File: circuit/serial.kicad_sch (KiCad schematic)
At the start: 21 parts, among them J1 Port B, J2 Port C, J4 Port A, J4 Port G, Q1 2N3904, Q2 2N3906, Q3 2N3906

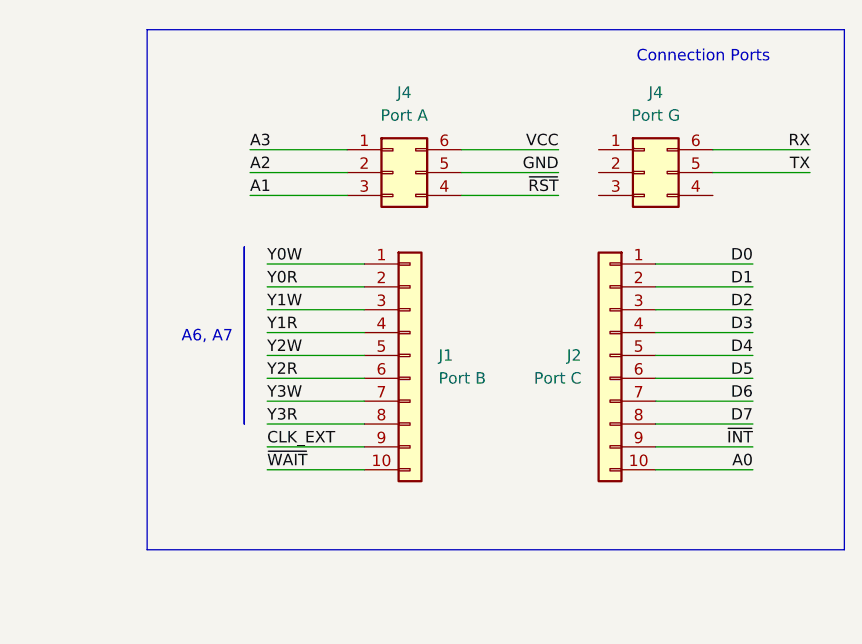
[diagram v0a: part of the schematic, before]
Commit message: .
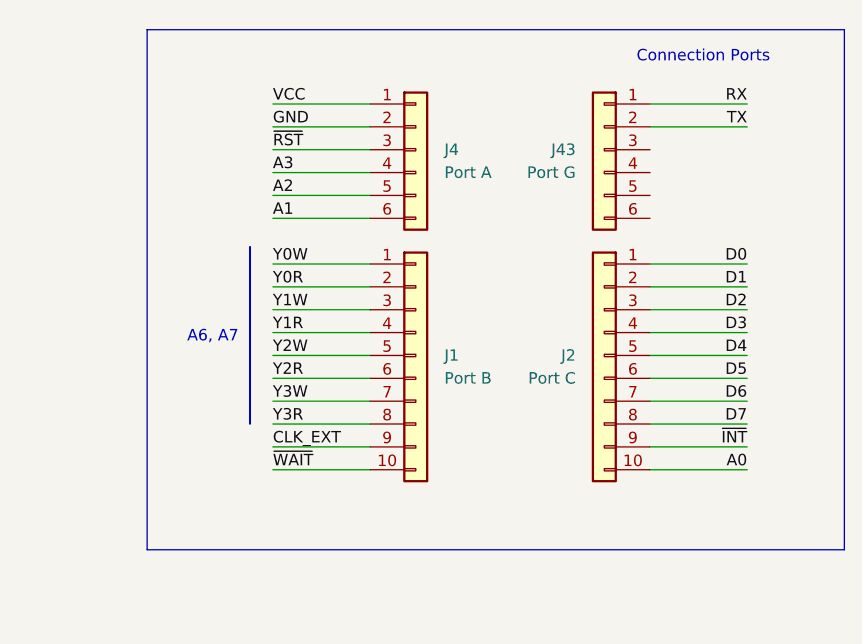
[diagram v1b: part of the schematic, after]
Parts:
- removed J4: Port A, symbol Connector_Generic:Conn_02x03_Counter_Clockwise
- removed J4: Port G, symbol Connector_Generic:Conn_02x03_Counter_Clockwise
- added J4: Port A, symbol Connector_Generic:Conn_01x06
- added J43: Port G, symbol Connector_Generic:Conn_01x06
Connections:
- net A1: now also J4.6 (Pin_6)
- net A2: now also J4.5 (Pin_5)
- net A3: now also J4.4 (Pin_4)
- net GND: now also J4.2 (Pin_2)
- net RX: now also J43.1 (Pin_1)
- net TX: now also J43.2 (Pin_2)
- net VCC: now also J4.1 (Pin_1)
- net ~{RST}: now also J4.3 (Pin_3)
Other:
- moved on the sheet: J1, J2
